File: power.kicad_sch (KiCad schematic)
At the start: 34 parts, among them IC3 LP5912-3.3DRVR, U12 BQ24075RGT, U2 LP5907SNX-1.8/NOPB, U3 LP5907SNX-3.3/NOPB, U6 LP5907SNX-3.3/NOPB, U7 LP5907SNX-3.3/NOPB

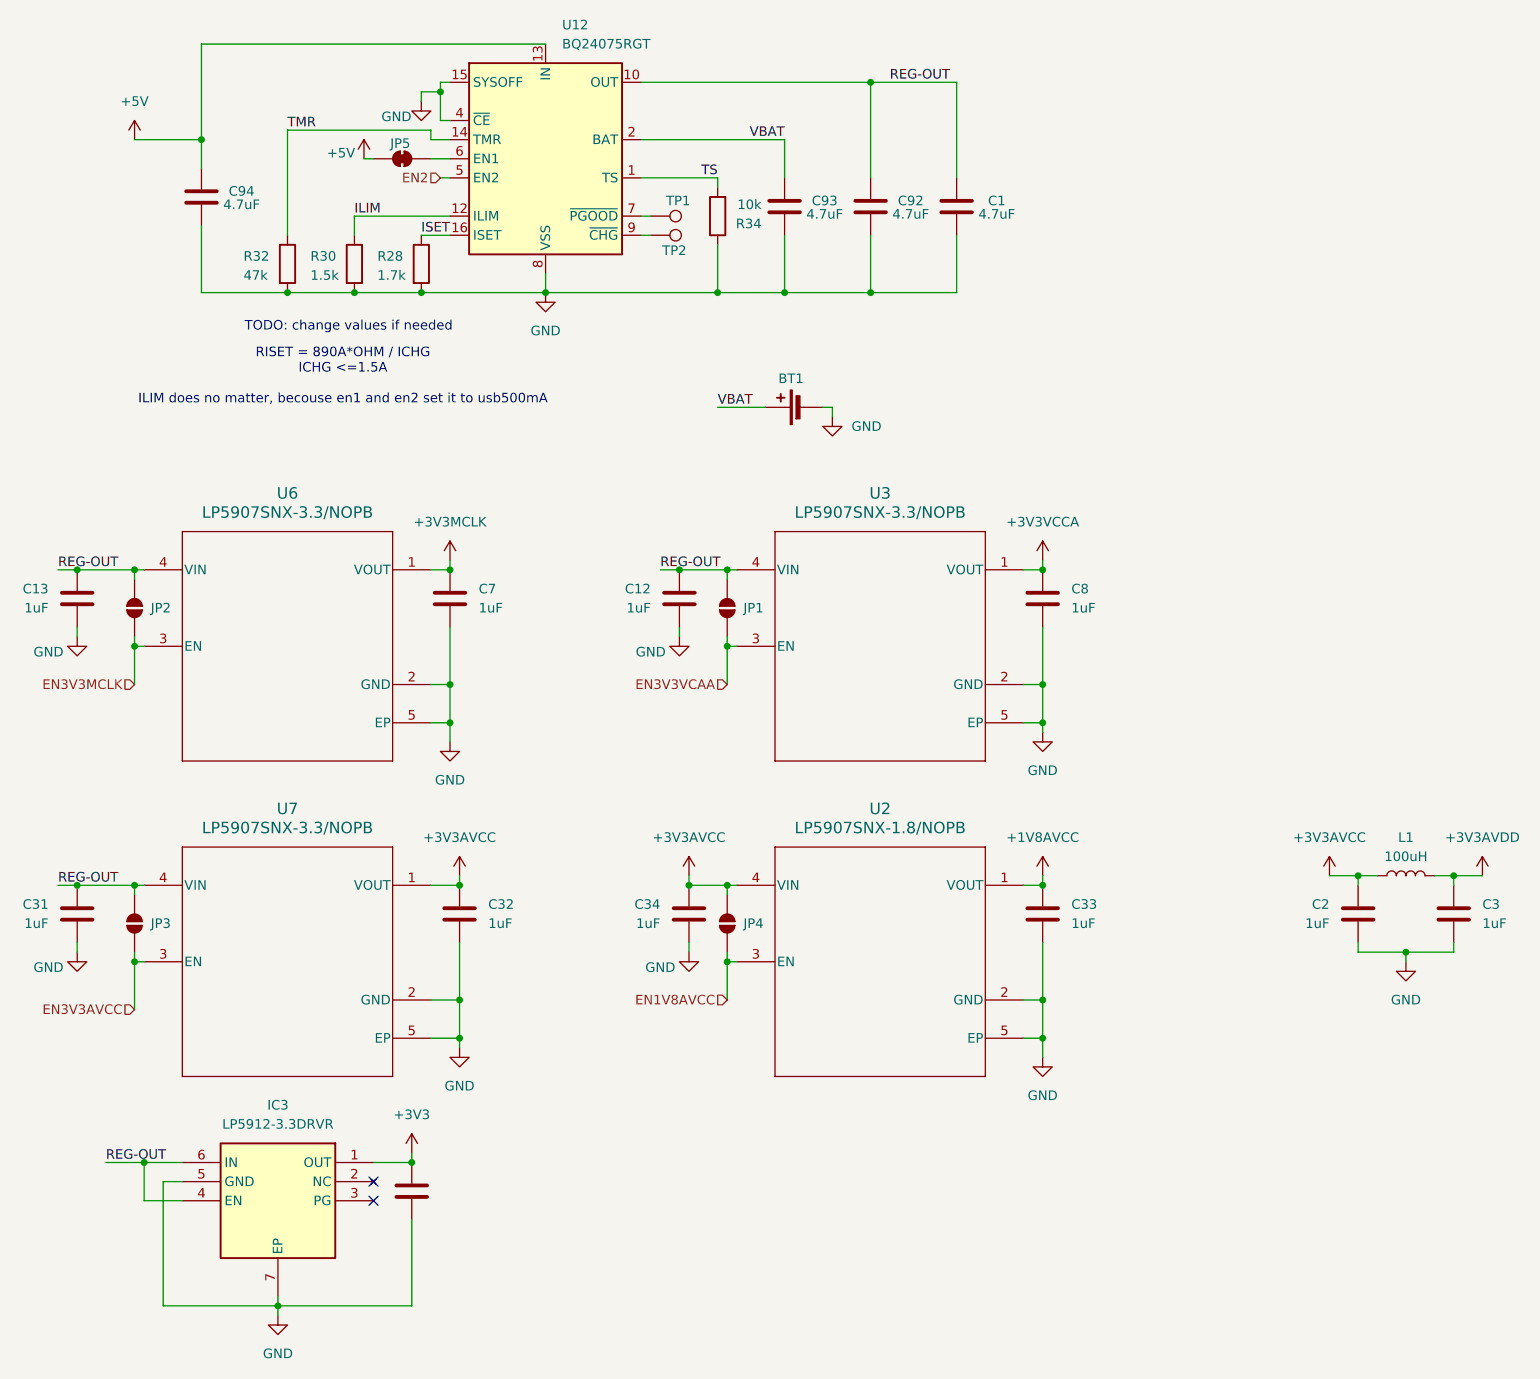
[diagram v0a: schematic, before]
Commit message: finishing up schematic
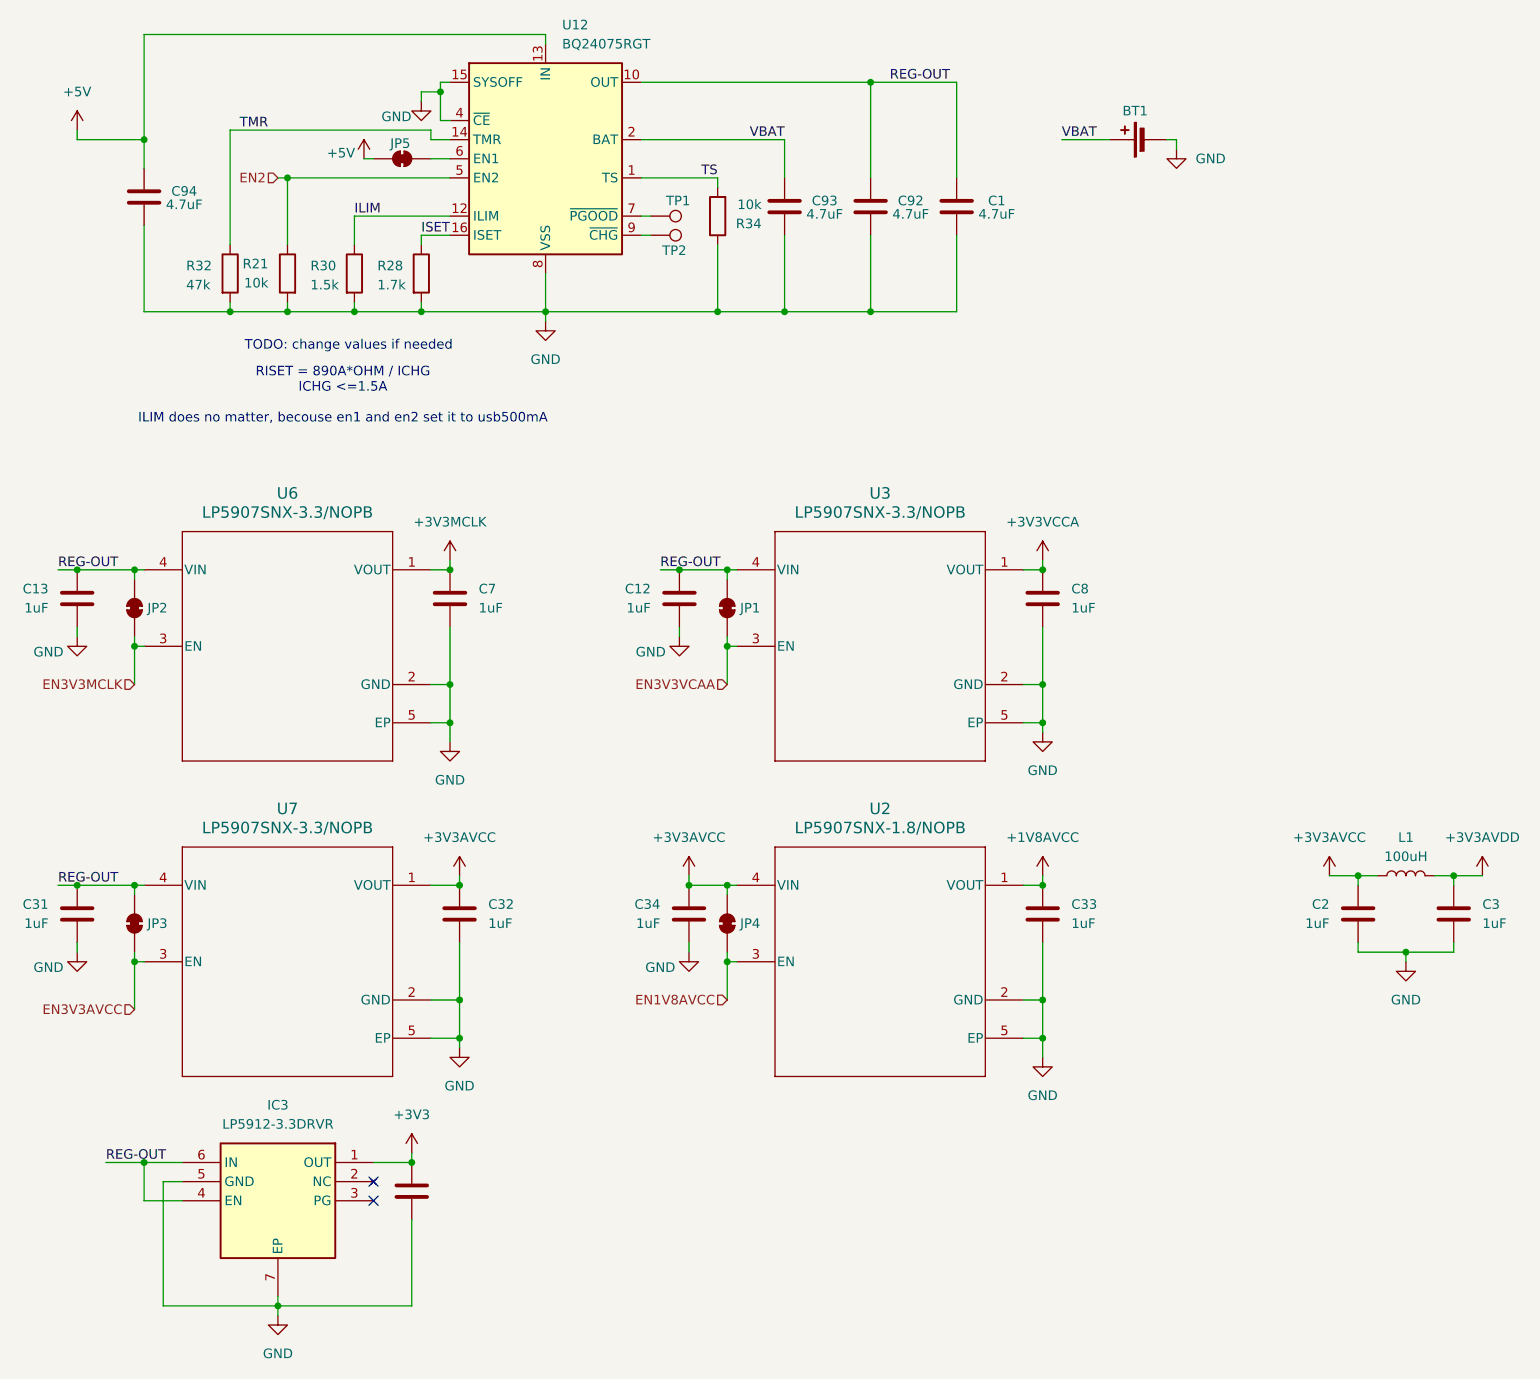
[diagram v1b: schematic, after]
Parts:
- removed JP1, JP2, JP3, JP4: SolderJumper_2_Open, Jumper:SolderJumper-2_P1.3mm_Open_RoundedPad1.0x1.5mm, symbol Jumper:SolderJumper_2_Open
- added JP1, JP2, JP3, JP4: SolderJumper_2_Bridged, Jumper:SolderJumper-2_P1.3mm_Bridged_RoundedPad1.0x1.5mm, symbol Jumper:SolderJumper_2_Bridged
- added R21: 10k, symbol Device:R
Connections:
- net +3V3AVCC: now also JP4.2 (B)
- net EN1V8AVCC: now also JP4.1 (A)
- net EN2: now also R21.1
- net EN3V3AVCC: now also JP3.1 (A)
- net EN3V3MCLK: now also JP2.1 (A)
- net EN3V3VCAA: now also JP1.1 (A)
- net GND: now also R21.2
- net REG-OUT: now also JP1.2 (B), JP2.2 (B), JP3.2 (B)
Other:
- moved on the sheet: BT1, C94, R28, R30, R32
